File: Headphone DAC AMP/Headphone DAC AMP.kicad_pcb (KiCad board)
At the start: 4 copper layers, 95 parts, among them J1 2137160001, J2 M50-3551042, J4 PINHD_1x2_Male, U1 NCV8187AMTW090TAG, U11 ADP5071AREZ-R7, U2 XU316-1024-QF60B-C24, U6 MCP1727-1802xSN, U7 MCP1727-3302xSN, U8 W25Q16JVSNIQ, Y1 Crystal_GND24, Y2 LMK6CE049152CDLFR, Y3 ASDLJ-E-45.1584MHz

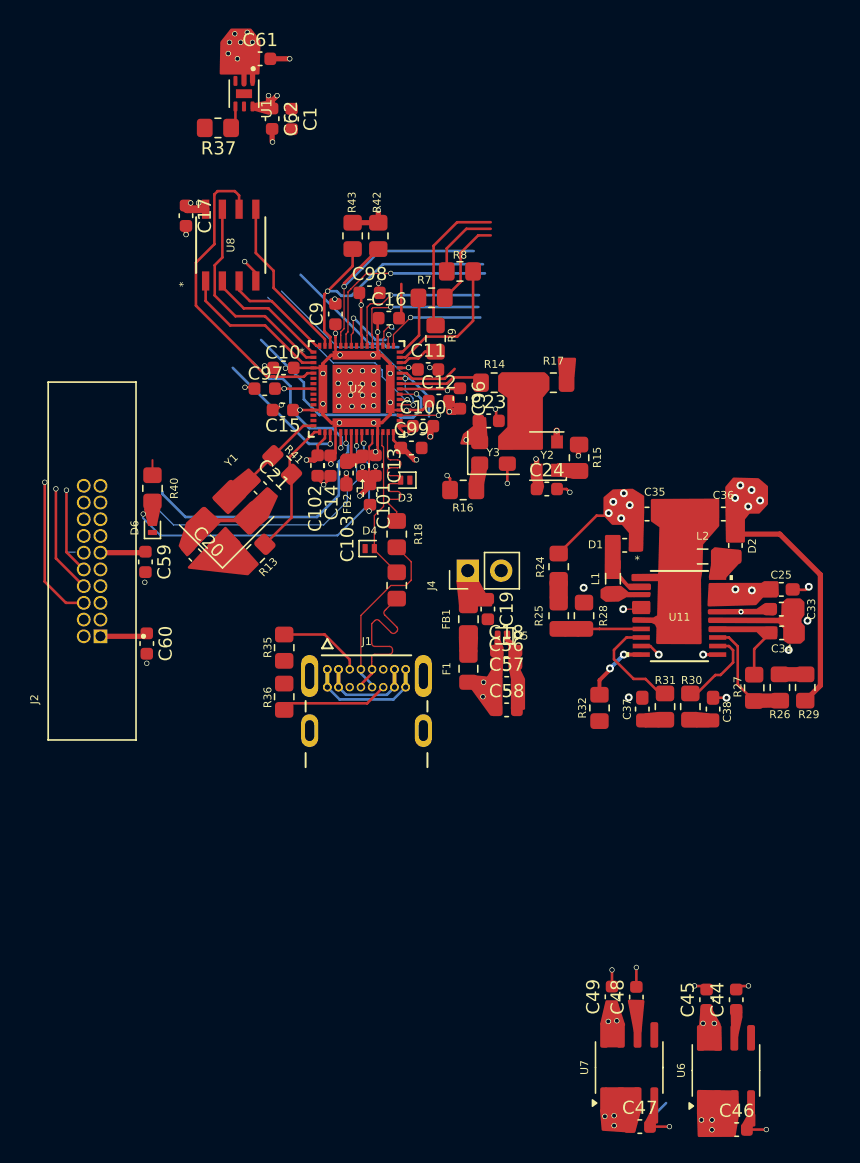
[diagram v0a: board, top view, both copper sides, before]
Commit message: Worked on layout briefley
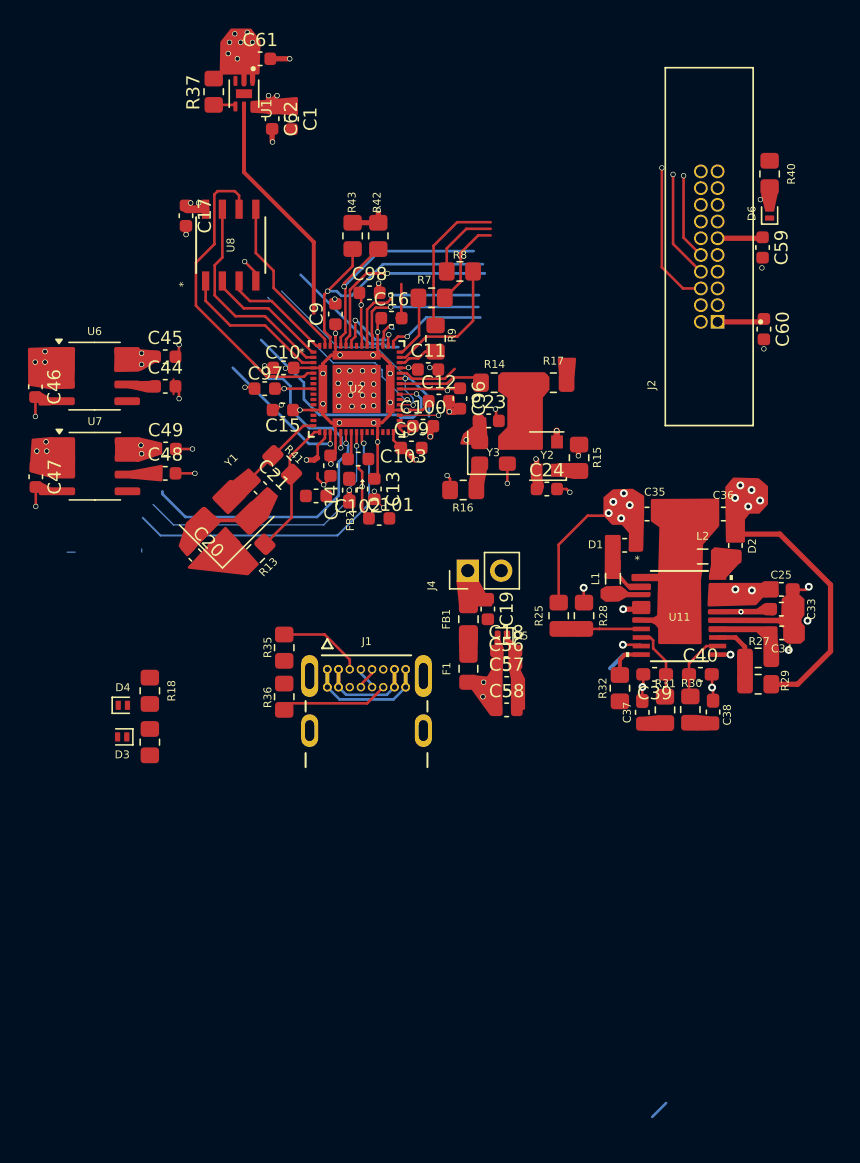
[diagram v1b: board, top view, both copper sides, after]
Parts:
- removed R24: 560K, Resistor_SMD:R_0805_2012Metric_Pad1.20x1.40mm_HandSolder
- removed R26: 36k, Resistor_SMD:R_0805_2012Metric_Pad1.20x1.40mm_HandSolder
- added C39: 22p, Capacitor_SMD:C_0603_1608Metric_Pad1.08x0.95mm_HandSolder, F.Cu at (119.7, 143.7)
- added C40: 39p, Capacitor_SMD:C_0603_1608Metric_Pad1.08x0.95mm_HandSolder, F.Cu at (123.2, 143.7)
- C37: value 47u -> 330p
- C38: value 47u -> 18n
- L1: value 3.3u -> 0.82u
- L2: value 4.7u -> 10u
- R25: value 100K -> 13K
- R27: value 100K -> 10.7k
- R28: value 27K -> 84.5K
- R29: value 750k -> 90.9k
- R30: value 4k -> 9.09k
- R31: value 1k -> 15k
- moved C46 77.6 mm to (72.7, 121.8), turned to -90 degrees
- moved U6 71.3 mm to (77.2, 121.0), turned to 0 degrees
- moved C47 67.4 mm to (72.7, 128.6), turned to -90 degrees
- moved C45 63.8 mm to (82.5, 119.5), turned to 0 degrees
- moved C44 63.6 mm to (82.5, 121.8), turned to 0 degrees
- moved U7 61.1 mm to (77.2, 127.8), turned to 0 degrees
- moved C49 53.7 mm to (82.6, 126.5), turned to 0 degrees
- moved C48 53.5 mm to (82.5, 128.4), turned to 0 degrees
- moved C59 52.6 mm to (127.9, 111.2)
- moved C60 52.6 mm to (128.0, 117.4)
- moved D6 52.6 mm to (128.4, 108.6)
- moved J2 52.6 mm to (123.9, 111.2)
- moved R40 52.6 mm to (128.4, 105.6)
- moved D3 29.0 mm to (79.3, 148.4)
- moved D4 22.2 mm to (79.3, 146.0)
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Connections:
- net /General Power/-5V5 renamed /General Power/-6V
- C35 pad 2: /General Power/+5V5 -> /General Power/+6V
- D1 pad 1: /General Power/+5V5 -> /General Power/+6V
- R28 pad 1: Net-(R24-Pad2) -> /General Power/+6V
- R29 pad 2: Net-(R26-Pad1) -> Net-(U11-FB2)
- U1 pad 6: +3.3V -> 0V9
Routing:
- net 0V9: track 39.8 -> 59.3 mm
- net /USB Audio Input/PRED+: track 13.9 -> 1.90 mm
- net /USB Audio Input/PRED-: track 13.9 -> 1.98 mm
- net /USB Audio Input/D+: track 11.7 -> 0.10 mm
- net /USB Audio Input/D-: track 11.7 -> 0.20 mm
- net /General Power/+6V: track 0.00 -> 10.5 mm, vias 0 -> 5
- net /General Power/+5V5: track 6.42 -> 0.00 mm, vias 5 -> 0
- net GND: track 51.9 -> 57.3 mm, vias 50 -> 49
- net /General Power/VREF: track 3.68 -> 0.00 mm
- net Net-(U11-FB2): track 6.47 -> 3.20 mm
- net Net-(U11-COMP1): track 8.12 -> 6.09 mm
- net /General Power/-6V: track 17.8 -> 19.4 mm
- net +1V8: track 39.1 -> 37.9 mm
- net +3.3V: track 45.7 -> 44.9 mm
- net Net-(U11-SS): track 5.14 -> 4.42 mm, vias 2 -> 0
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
